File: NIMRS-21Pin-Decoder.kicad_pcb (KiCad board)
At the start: 4 copper layers, 30 x 15.5 mm, 75 parts, among them J1 21Pin Loco Socket, J2 U.FL, Q1 MMDT3904, Q2 MMDT3904, U1 ESP32-S3FN8, U2 MAX98357A, U4 DRV8213DSGR, U60 TPS63070, U70 TPS63070, X1 40Mhz

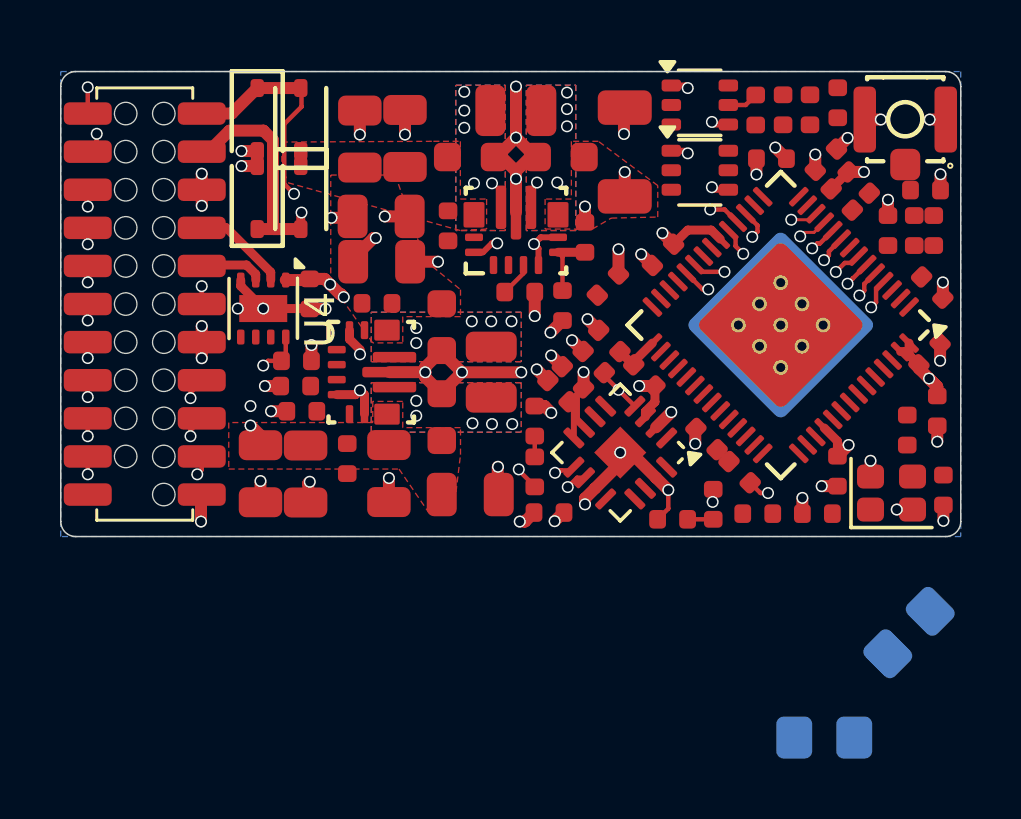
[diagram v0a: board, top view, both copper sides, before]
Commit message: PCB Checkpoint
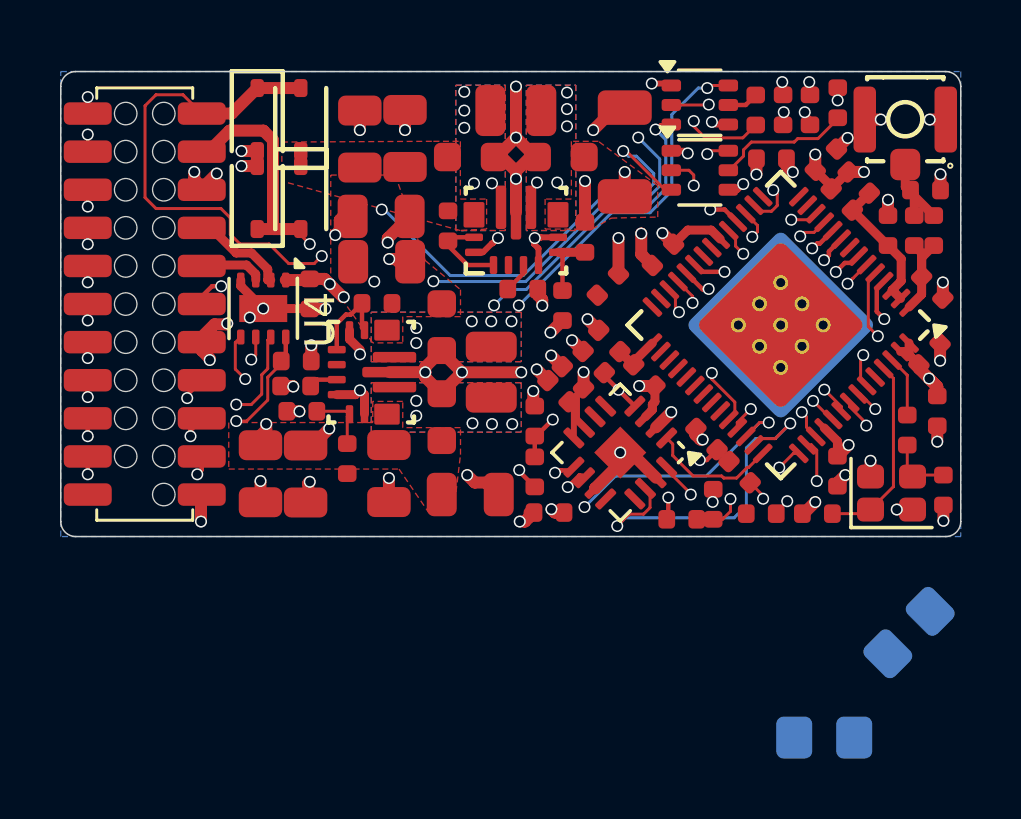
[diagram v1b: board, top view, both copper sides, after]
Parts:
- moved R7 0.30 mm to (20.7, 14.9)
- moved C76 0.14 mm to (15.4, 7.25)
- moved R1 0.12 mm to (23.4, 14.7)
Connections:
- U1 pad 38: /AUX3 -> /AMP_SD_MODE
- U1 pad 40: /VMOTOR_PG -> /AUX3
- U1 pad 41: /AMP_SD_MODE -> /AMP_LRCLK
- U1 pad 44: /AMP_LRCLK -> /VMOTOR_PG
- U1 pad 6: /MOTOR_CURRENT -> /TRACK_RIGHT
- U1 pad 9: /TRACK_RIGHT -> /MOTOR_CURRENT
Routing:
- net /rear: track 0.53 -> 32.6 mm, vias 1 -> 3
- net /front: track 0.56 -> 31.1 mm, vias 1 -> 3
- net /aux1: track 0.75 -> 30.7 mm, vias 1 -> 4
- net /aux2: track 0.75 -> 28.9 mm, vias 1 -> 3
- net /AUX4: track 1.52 -> 27.6 mm
- net /ZBDTA/D+: track 0.54 -> 26.5 mm, vias 1 -> 2
- net /ZBCLK/D-: track 0.54 -> 26.2 mm, vias 1 -> 2
- net /AUX3: track 0.66 -> 24.2 mm, vias 1 -> 3
- net /+V_SENSE: track 1.62 -> 19.3 mm, vias 1 -> 2
- net /VMOTOR_PG: track 0.60 -> 14.5 mm, vias 1 -> 2
- net /AUX5: track 1.55 -> 15.2 mm
- net /AMP_LRCLK: track 0.00 -> 11.9 mm, vias 0 -> 2
- net /TRACK_LEFT: track 1.52 -> 13.2 mm, vias 1 -> 2
- net /TRACK_RIGHT: track 1.79 -> 12.4 mm, vias 1 -> 2
- net /FRONT: track 0.00 -> 8.70 mm, vias 0 -> 2
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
